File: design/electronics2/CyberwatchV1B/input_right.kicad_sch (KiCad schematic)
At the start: 0 parts

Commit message: electronics progres
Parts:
- added J8: Conn_01x07_main, symbol Connector_Generic:Conn_01x07
- added SW4: SW_Push, Button_Switch_SMD:SW_Push_1P1T_NO_CK_KMR2, symbol Switch:SW_Push
- added U5: MT6701CT, Package_SO:SO-8_3.9x4.9mm_P1.27mm, symbol Sensor_Magnetic:MT6701CT
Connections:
- new net +3.3V: U5.1 (VDD)
- new net BTN_3: U5.5 (PUSH)
- new net BTN_4: SW4.2
- new net GND: SW4.1, U5.2 (MODE), U5.4 (GND)
- new net SCL: U5.7 (B)
- new net SDA: U5.6 (A)
- no-connect marks 0 -> 2

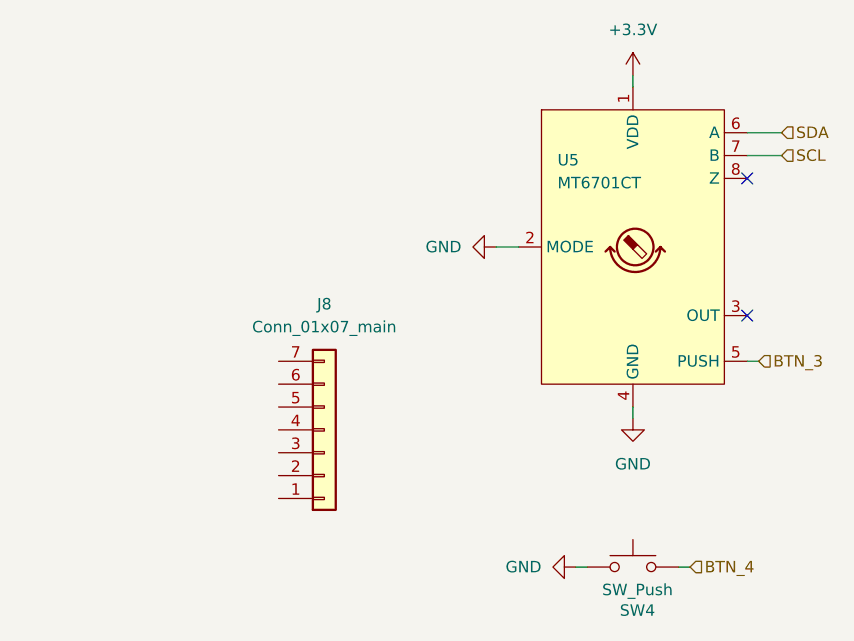
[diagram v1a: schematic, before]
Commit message: schematic complete
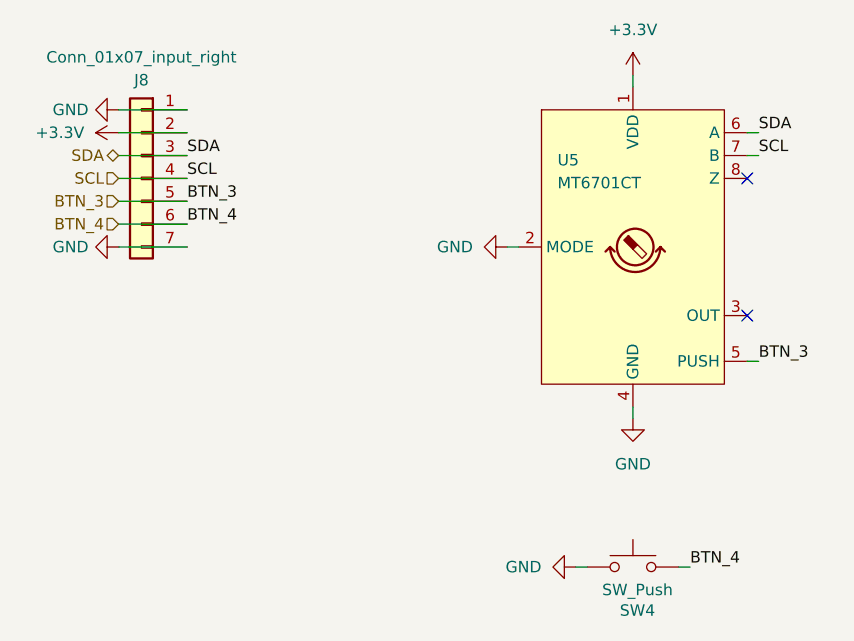
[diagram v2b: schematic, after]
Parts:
- J8: value Conn_01x07_main -> Conn_01x07_input_right
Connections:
- net +3.3V: now also J8.2 (Pin_2)
- net BTN_3: now also J8.5 (Pin_5)
- net BTN_4: now also J8.6 (Pin_6)
- net GND: now also J8.1 (Pin_1), J8.7 (Pin_7)
- net SCL: now also J8.4 (Pin_4)
- net SDA: now also J8.3 (Pin_3)
